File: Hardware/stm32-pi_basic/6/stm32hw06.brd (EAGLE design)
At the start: 73.1 x 74 mm, 74 parts, among them IC1 CP2102, J1 CONN_12X2, U1 ESP32-WROOM-32D

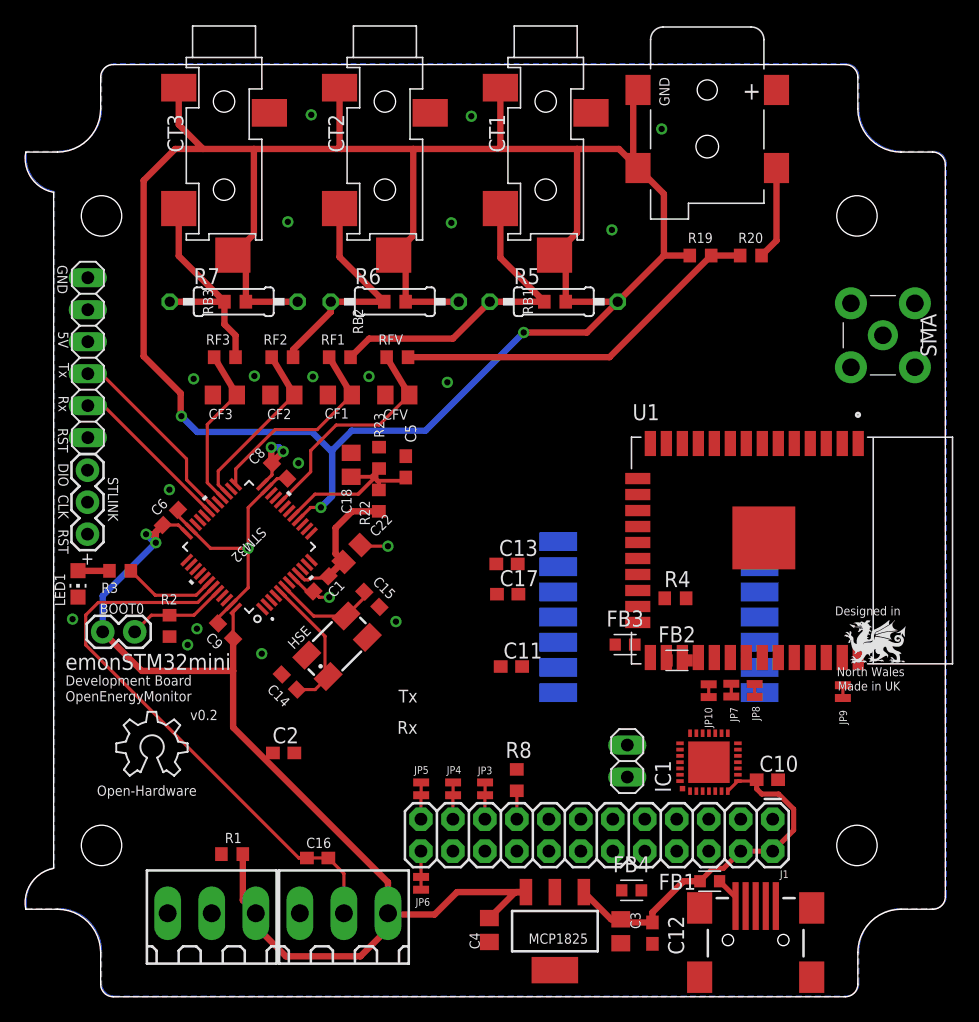
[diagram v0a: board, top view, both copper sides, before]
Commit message: sync mini v0.2
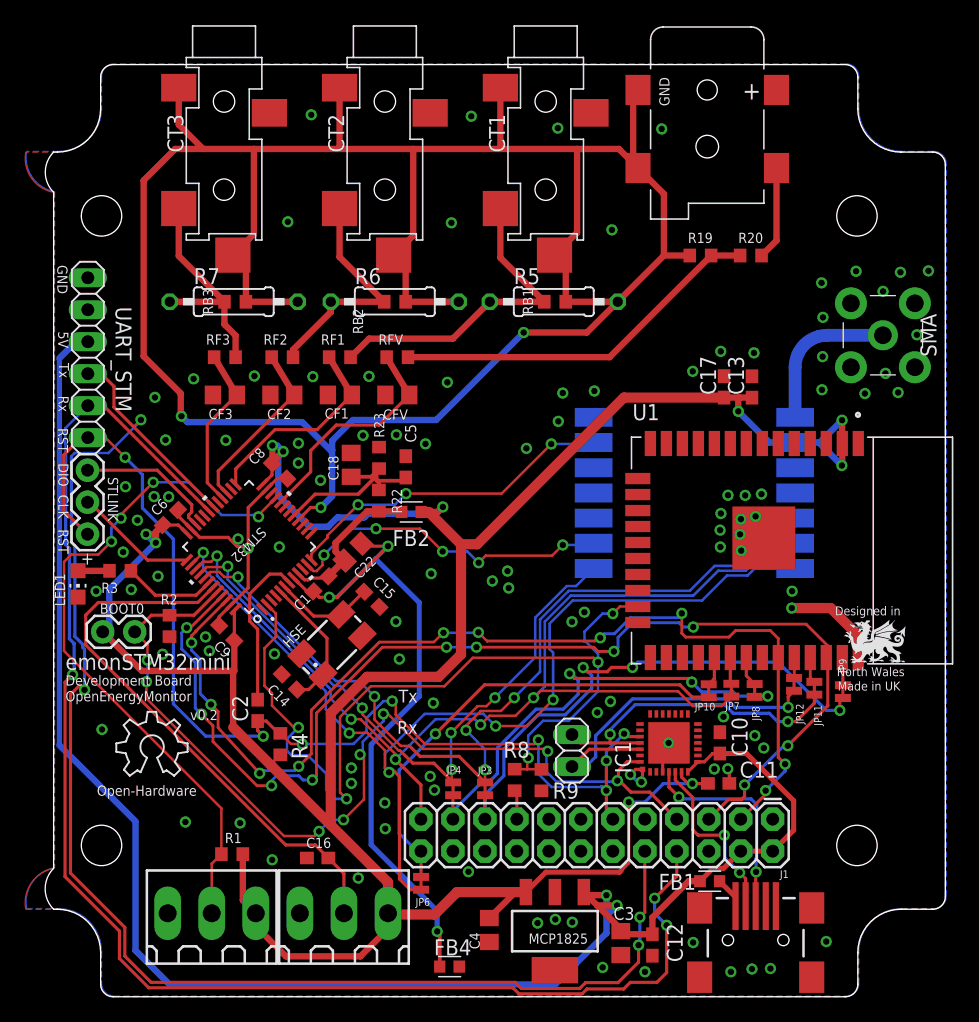
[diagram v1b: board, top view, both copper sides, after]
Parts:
- removed FB3: FBCHIP-0603(1608-METRIC), Filter:BEADC1608X95N
- removed JP5: JUMPER-SMT_2_NC_TRACE_NO-SILK, SparkFun-Jumpers:SMT-JUMPER_2_NC_TRACE_NO-SILK
- added JP11, JP12: JUMPER-SMT_2_NC_TRACE_NO-SILK, SparkFun-Jumpers:SMT-JUMPER_2_NC_TRACE_NO-SILK
- added R9: 10k, rcl:R0603
- C2: value 100nF -> 2.2uF
- R8: value 10k -> 120k
- moved R4 33.4 mm to (25.5, 26.4), turned to 270 degrees
- moved FB2 24.2 mm to (35.9, 44.8), turned to 180 degrees
- moved C13 24.0 mm to (63.0, 54.7), turned to 90 degrees
- moved C17 23.8 mm to (60.8, 54.7), turned to 90 degrees
- moved C11 18.9 mm to (60.3, 23.2)
- moved FB4 15.7 mm to (39.0, 8.68)
- moved U$2 10.3 mm to (60.4, 45.3)
- moved C10 4.78 mm to (60.4, 26.5), turned to 90 degrees
- moved JP1 4.47 mm to (48.7, 25.8), turned to 270 degrees
- moved C2 3.96 mm to (23.7, 29.0), turned to 90 degrees
- moved IC1 3.52 mm to (56.4, 26.4)
- moved C12 0.94 mm to (55.1, 10.4)
- moved C3 0.94 mm to (52.6, 10.5)
- moved HSE 0.42 mm to (29.6, 34.2)
- moved C9 0.18 mm to (21.3, 35.2)
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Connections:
- removed net GND_USB: FB3.2, U$10.GND, U$10.MTN1, U$10.MTN2, U$10.MTN3, U$10.MTN4
- removed net MISO_RPI: J1.21, JP4.2
- removed net MOSI_RPI: J1.19, JP3.2
- removed net RPI_CLK: J1.23, JP5.2, JP7.2
- removed net SPI3_CLK: JP5.1, STM32.39, U$2.13
- removed net UART_RX: IC1.26, JP1.1
- removed net UART_TX: IC1.25, JP1.2
- new net CP2102_RX: IC1.25, JP1.1, JP11.1
- new net CP2102_TX: IC1.26, JP1.2, JP12.1
- new net SPI_CLK: J1.23, JP7.2, STM32.39, U$2.13
- net ESP_RX: now also JP12.2
- net ESP_TX: now also JP11.2
- net GND: now also R9.1, U$10.GND, U$10.MTN1, U$10.MTN2, U$10.MTN3, U$10.MTN4; no longer FB3.1
- net NRST: no longer STLINK.3
- net RPI_CONNECTED: now also R9.2
- net RPI_MISO: now also J1.21, JP4.2
- net RPI_MOSI: now also J1.19, JP3.2
- net RST_STM: now also STLINK.3
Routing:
- net +3V3: track 97.3 -> 220.7 mm, vias 4 -> 10
- net +5V: track 29.8 -> 135.1 mm, vias 0 -> 2
- net STM_RX: track 13.1 -> 116.2 mm, vias 0 -> 3
- net STM_TX: track 15.3 -> 117.8 mm, vias 0 -> 4
- net SCL: track 0.00 -> 93.9 mm, vias 0 -> 10
- net SPI_CLK: track 0.00 -> 89.2 mm, vias 0 -> 5
- net RST_STM: track 0.00 -> 88.6 mm, vias 0 -> 8
- net SDA: track 0.00 -> 84.4 mm, vias 0 -> 10
- net SPI3_NSS: track 0.00 -> 82.2 mm, vias 0 -> 5
- net RPI_CONNECTED: track 0.00 -> 72.5 mm, vias 0 -> 5
- net SPI3_MOSI: track 0.00 -> 72.0 mm, vias 0 -> 5
- net BOOT0: track 7.94 -> 75.2 mm, vias 0 -> 8
- net DS18B20: track 0.00 -> 55.5 mm, vias 0 -> 4
- net SPI3_MISO: track 0.00 -> 50.9 mm, vias 0 -> 5
- net AGND: track 5.68 -> 56.0 mm, vias 2 -> 3
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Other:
- board size 73.1 x 74 mm -> 71.5 x 74 mm
